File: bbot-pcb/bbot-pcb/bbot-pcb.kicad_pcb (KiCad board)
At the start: 2 copper layers, 66 x 54.6 mm, 11 parts, among them U1 HA-552-4P, U3 HA-552-4P

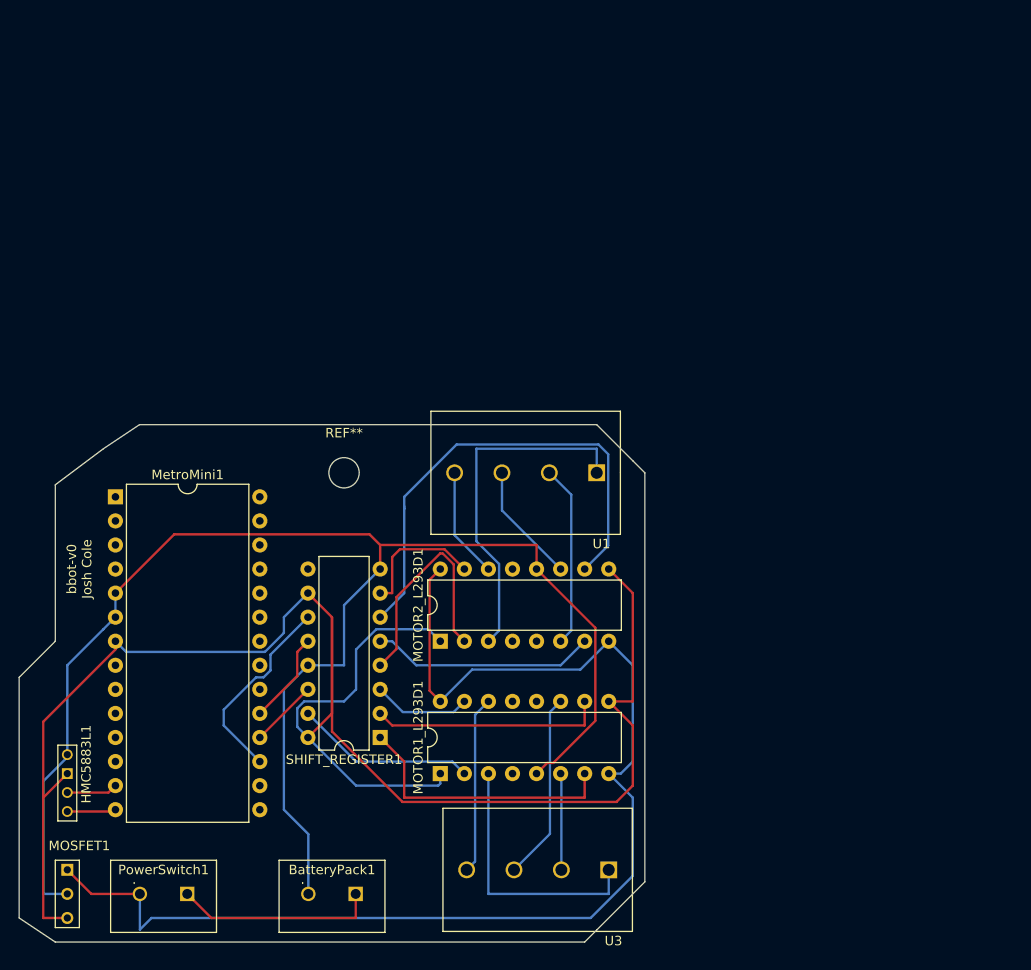
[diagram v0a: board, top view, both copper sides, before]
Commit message: pcb v2 updates
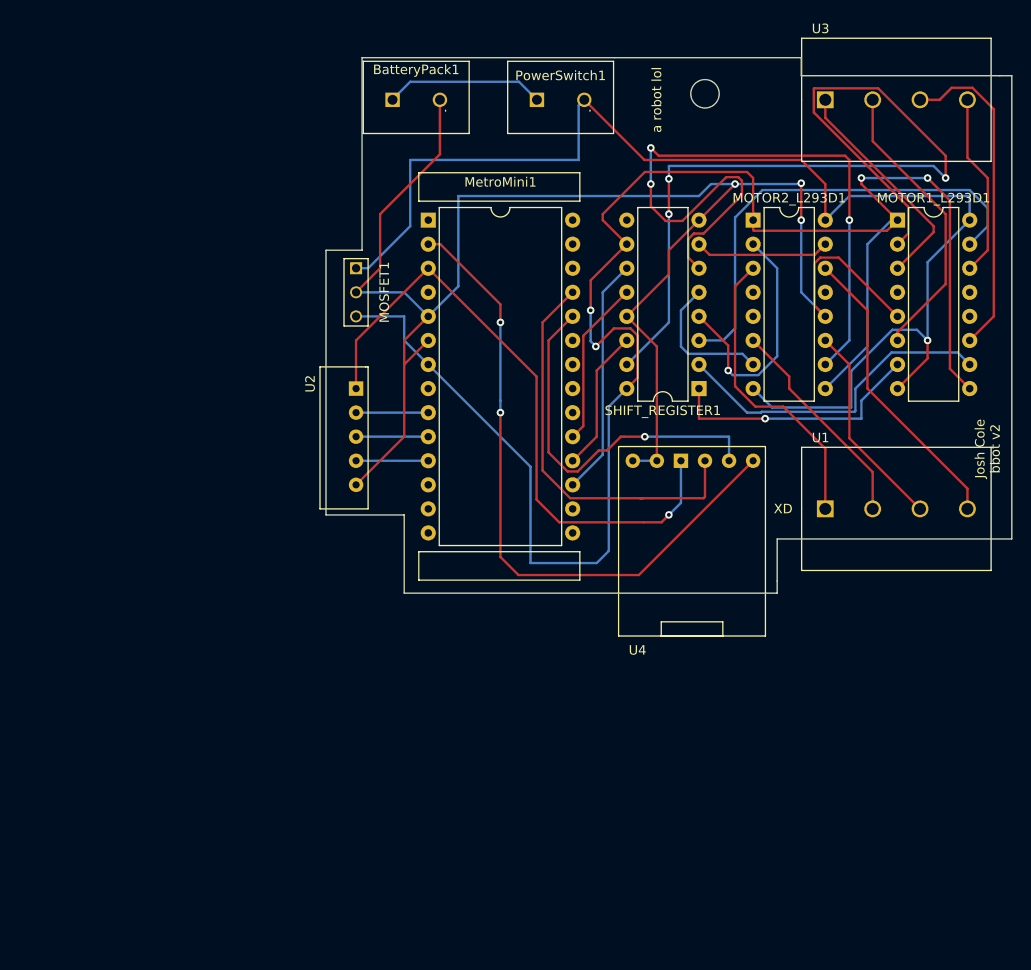
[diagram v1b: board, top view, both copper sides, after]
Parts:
- removed HMC5883L1: HMC5883L, bbot-pcb:HMC588L
- removed the REF** at (146.1, 62.2)
- added REF**: MountingHole_3mm, MountingHole:MountingHole_3mm, F.Cu at (184.2, 22.2)
- added U2: ADXL335, bbot-pcb:ADXL335, F.Cu at (147.3, 53.3)
- added U4: OPENLOG, bbot-pcb:OPENLOG, F.Cu at (176.5, 61.0)
- moved PowerSwitch1 93.7 mm to (168.9, 22.9), turned to 0 degrees
- moved U3 84.4 mm to (196.8, 22.9), turned to 0 degrees
- moved BatteryPack1 84.3 mm to (153.7, 22.9), turned to 0 degrees
- moved MOTOR1_L293D1 75.8 mm to (204.5, 35.6), turned to 0 degrees
- moved MOSFET1 70.4 mm to (147.3, 43.2)
- moved MOTOR2_L293D1 55.4 mm to (189.2, 35.6), turned to 0 degrees
- moved SHIFT_REGISTER1 49.9 mm to (183.5, 53.3)
- moved MetroMini1 44.1 mm to (154.9, 35.6)
- moved U1 24.4 mm to (196.8, 66.0), turned to 0 degrees
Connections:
- MetroMini1 pad 10: Net-(MetroMini1-Pad10) -> /A1
- MetroMini1 pad 11: Net-(MetroMini1-Pad11) -> /A2
- MetroMini1 pad 2: Net-(MetroMini1-Pad2) -> /RST
- MetroMini1 pad 24: Net-(MetroMini1-Pad24) -> /RX
- MetroMini1 pad 25: Net-(MetroMini1-Pad25) -> /TX
- MetroMini1 pad 3: Net-(MetroMini1-Pad3) -> /3V
- MetroMini1 pad 9: Net-(MetroMini1-Pad9) -> /A0
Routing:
- net /MOTOR1_A: track 19.1 -> 92.9 mm, vias 0 -> 3
- net /RST: track 0.00 -> 69.4 mm, vias 0 -> 2
- net /3V: track 0.00 -> 66.5 mm, vias 0 -> 1
- net /TX: track 0.00 -> 42.7 mm
- net /RX: track 0.00 -> 39.4 mm, vias 0 -> 1
- net /MOTOR1_D: track 10.3 -> 49.3 mm
- net /MOTOR2_C: track 51.4 -> 75.3 mm, vias 0 -> 3
- net /MOTOR1_PHASE_B: track 10.2 -> 30.7 mm
- net /MOTOR2_PHASE_D: track 11.6 -> 31.6 mm
- net GND: track 158.9 -> 178.6 mm, vias 0 -> 3
- net /MOTOR1_PHASE_C: track 19.8 -> 34.7 mm
- net /MOTOR1_C: track 24.7 -> 35.2 mm
- net /MOTOR2_PHASE_C: track 12.7 -> 21.9 mm
- net /MOTOR2_B: track 23.7 -> 14.9 mm
- net 5V: track 197.6 -> 189.3 mm, vias 0 -> 4
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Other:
- board size 66 x 54.6 mm -> 72.4 x 56.5 mm
- board text added: "Josh Cole bbot v2"
- board text added: "XD"
- board text added: "a robot lol"
- board text removed: "Battery Pack"
- board text removed: "Power Switch"
- board text removed: "a robot"
- board text removed: "bbot-v0 Josh Cole"
- board text removed: "is this enough?"
- board text removed: "lol"
